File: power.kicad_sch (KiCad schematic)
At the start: 29 parts, among them U17 TPS62933, U6 TLV62569DBV, U9 TPS2121RUXR

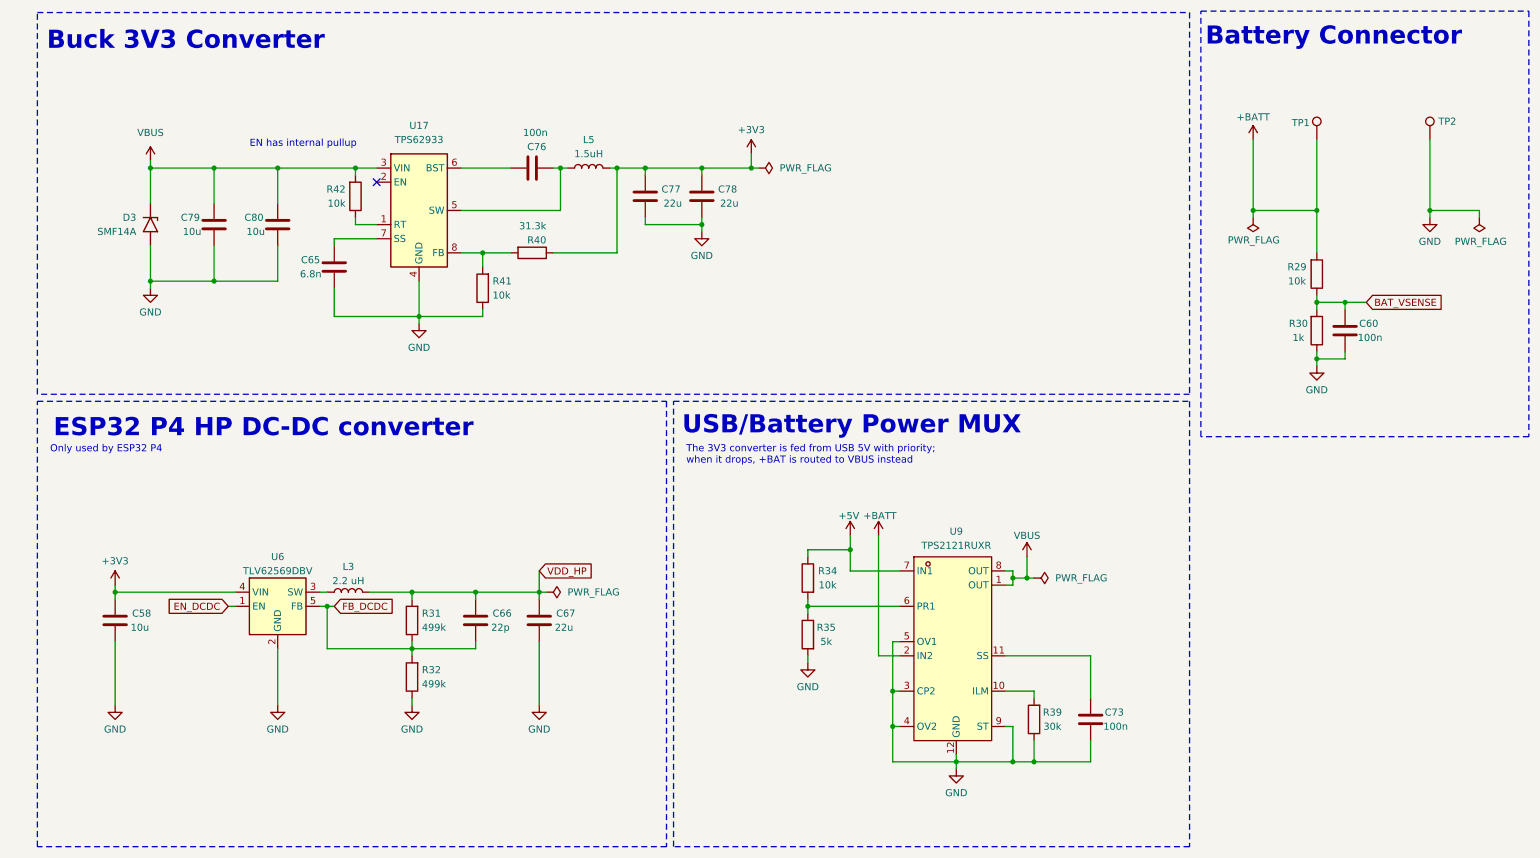
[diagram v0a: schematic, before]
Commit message: Good placement of most FC components
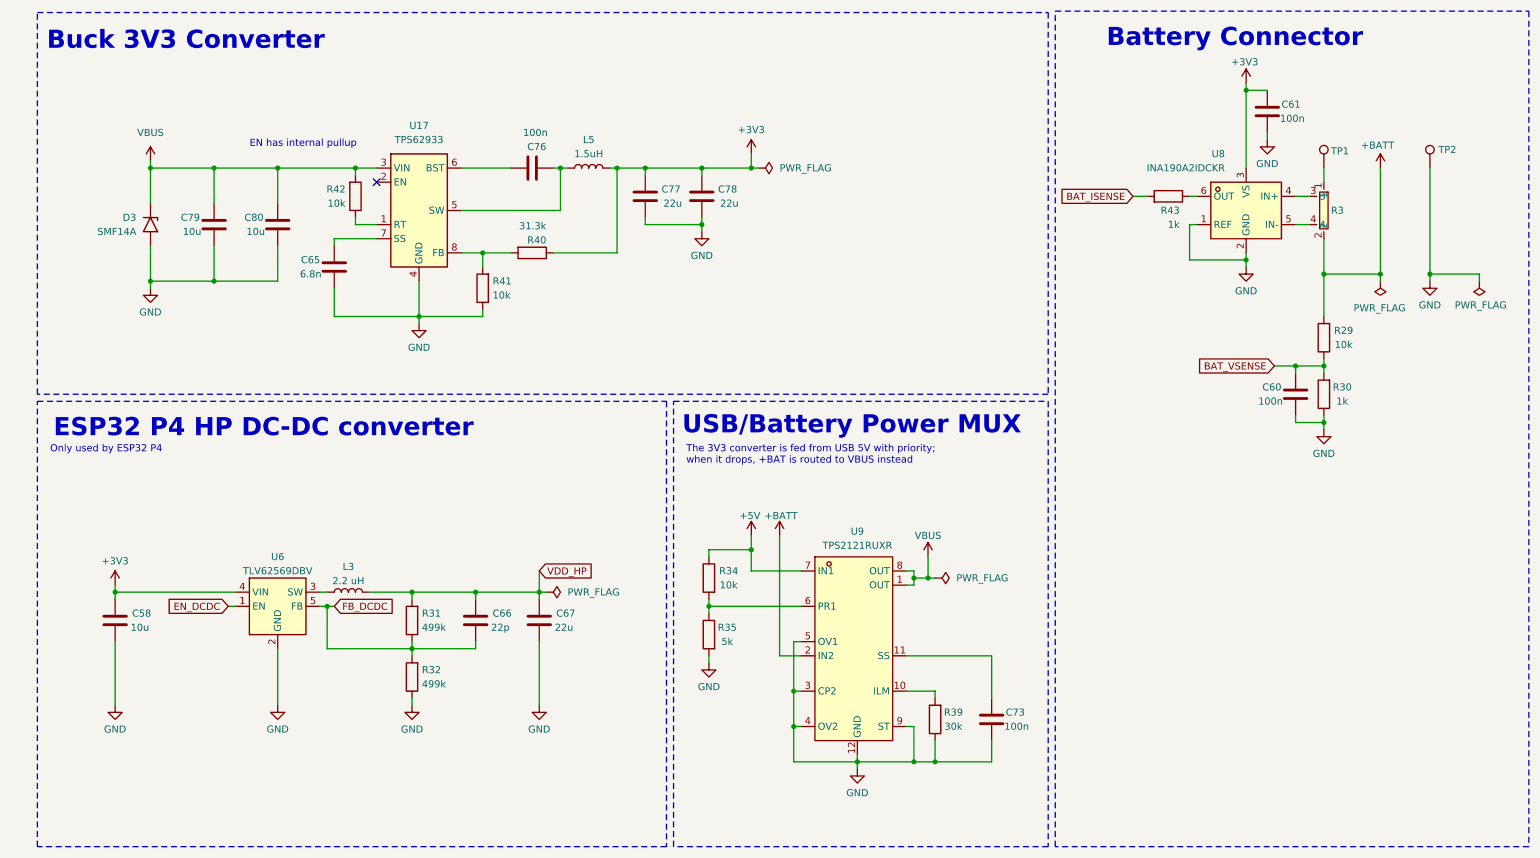
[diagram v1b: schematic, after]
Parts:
- added C61: 100n, Capacitor_SMD:C_0201_0603Metric, symbol Device:C
- added R3: BVN-Z-R0005-1.0, easyeda2kicad:RES-SMD_4P-L4.1-W3.1-BL_BVN-1216, symbol easyeda2kicad:BVN-Z-R0005-1.0
- added R43: 1k, Resistor_SMD:R_0201_0603Metric, symbol Device:R
- added U8: INA190A2IDCKR, easyeda2kicad:SC-70-6_L2.0-W1.3-P0.65-LS2.1-BR, symbol easyeda2kicad:INA190A2IDCKR
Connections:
- net +3V3: now also C61.1, U8.3 (VS)
- net +BATT: now also R3.2; no longer TP1.1
- net GND: now also C61.2, U8.1 (REF), U8.2 (GND)
- new net: R3.3, U8.4 (IN+)
- new net: R3.4, U8.5 (IN-)
- new net: R43.1, U8.6 (OUT)
- new net: R3.1, TP1.1
- new net BAT_ISENSE: R43.2
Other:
- moved on the sheet: C60, C73, R29, R30, R34, R35, R39, TP1, TP2, U9
